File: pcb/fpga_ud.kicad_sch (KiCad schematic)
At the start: 1 part

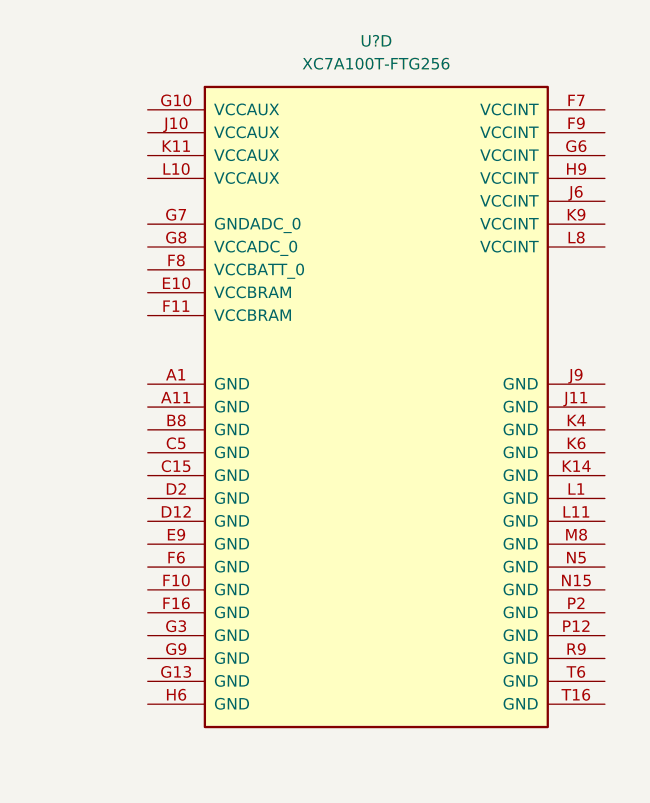
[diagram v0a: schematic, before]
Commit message: fpga shite
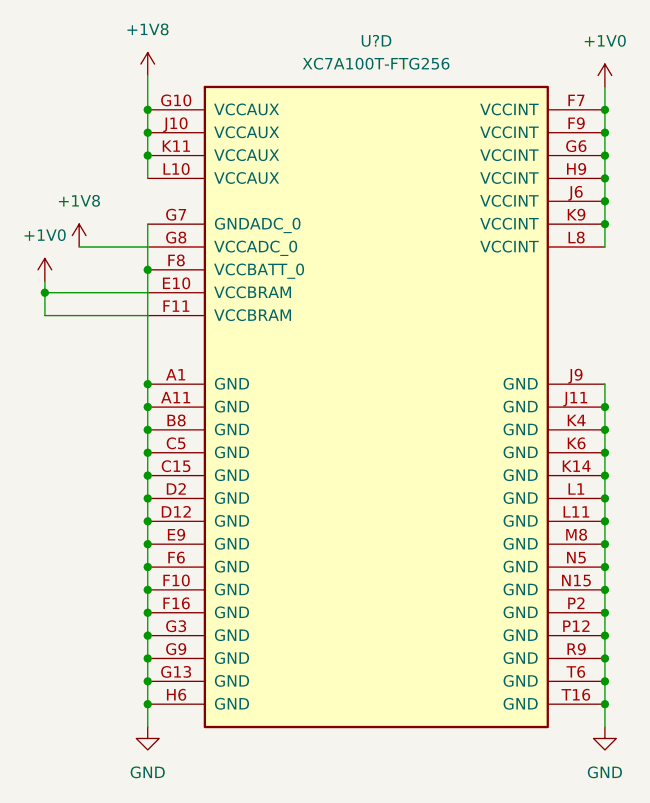
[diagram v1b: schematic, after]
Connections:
- net GND: now reaches U?.A1 (GND)
- net GND: now also U?.A11 (GND), U?.B8 (GND), U?.C15 (GND), U?.C5 (GND), U?.D12 (GND), U?.D2 (GND), U?.E9 (GND), U?.F10 (GND), U?.F16 (GND), U?.F6 (GND), U?.F8 (VCCBATT_0), U?.G13 (GND), U?.G3 (GND), U?.G7 (GNDADC_0), U?.G9 (GND), U?.H6 (GND), U?.J11 (GND), U?.J9 (GND), U?.K14 (GND), U?.K4 (GND), U?.K6 (GND), U?.L1 (GND), U?.L11 (GND), U?.M8 (GND), U?.N15 (GND), U?.N5 (GND), U?.P12 (GND), U?.P2 (GND), U?.R9 (GND), U?.T16 (GND), U?.T6 (GND)
- net +1V0: now reaches U?.E10 (VCCBRAM)
- net +1V0: now also U?.F11 (VCCBRAM), U?.F7 (VCCINT), U?.F9 (VCCINT), U?.G6 (VCCINT), U?.H9 (VCCINT), U?.J6 (VCCINT), U?.K9 (VCCINT), U?.L8 (VCCINT)
- net +1V8: now reaches U?.G10 (VCCAUX)
- net +1V8: now also U?.G8 (VCCADC_0), U?.J10 (VCCAUX), U?.K11 (VCCAUX), U?.L10 (VCCAUX)
